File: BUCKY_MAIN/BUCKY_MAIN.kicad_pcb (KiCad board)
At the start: 2 copper layers, 190 x 162.2 mm, 17 parts, among them J2 MAG_CONN, J4 Conn_01x10, U1 IFX9201SG_BO, U2 IFX9201SG_BO, U3 IFX9201SG_BO, U9 PCA9548ADB

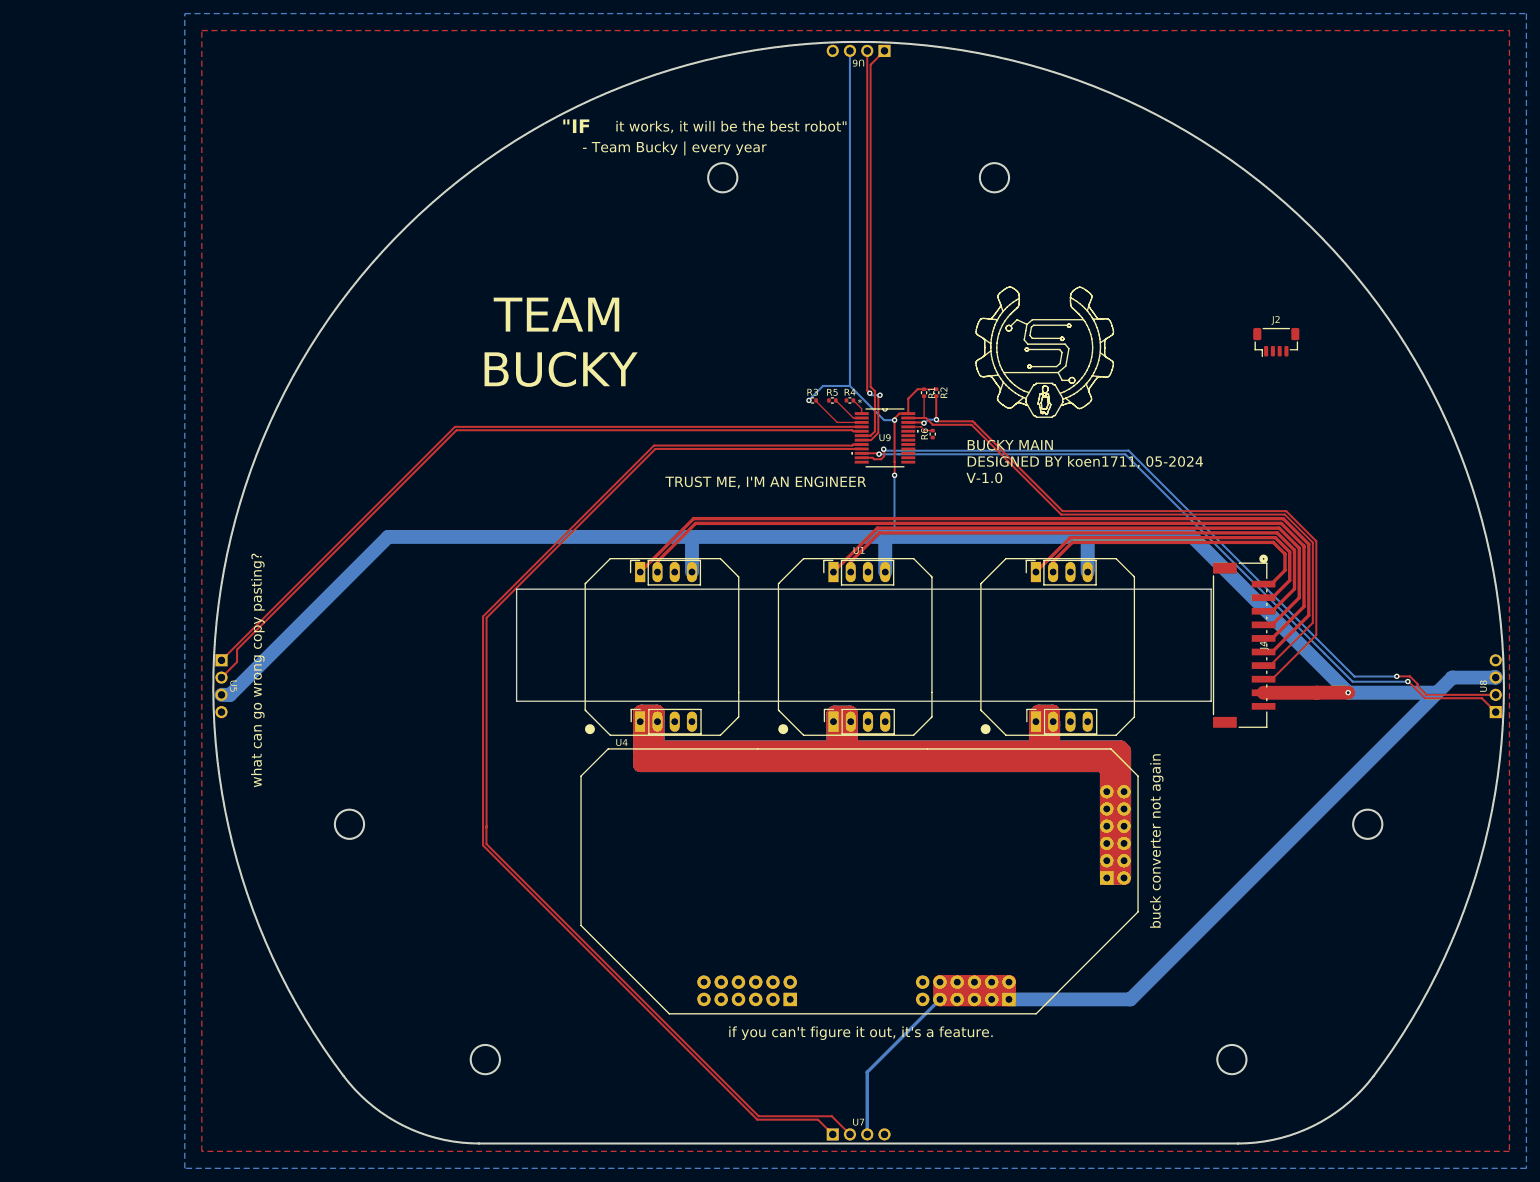
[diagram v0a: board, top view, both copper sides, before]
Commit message: chore: finish main board
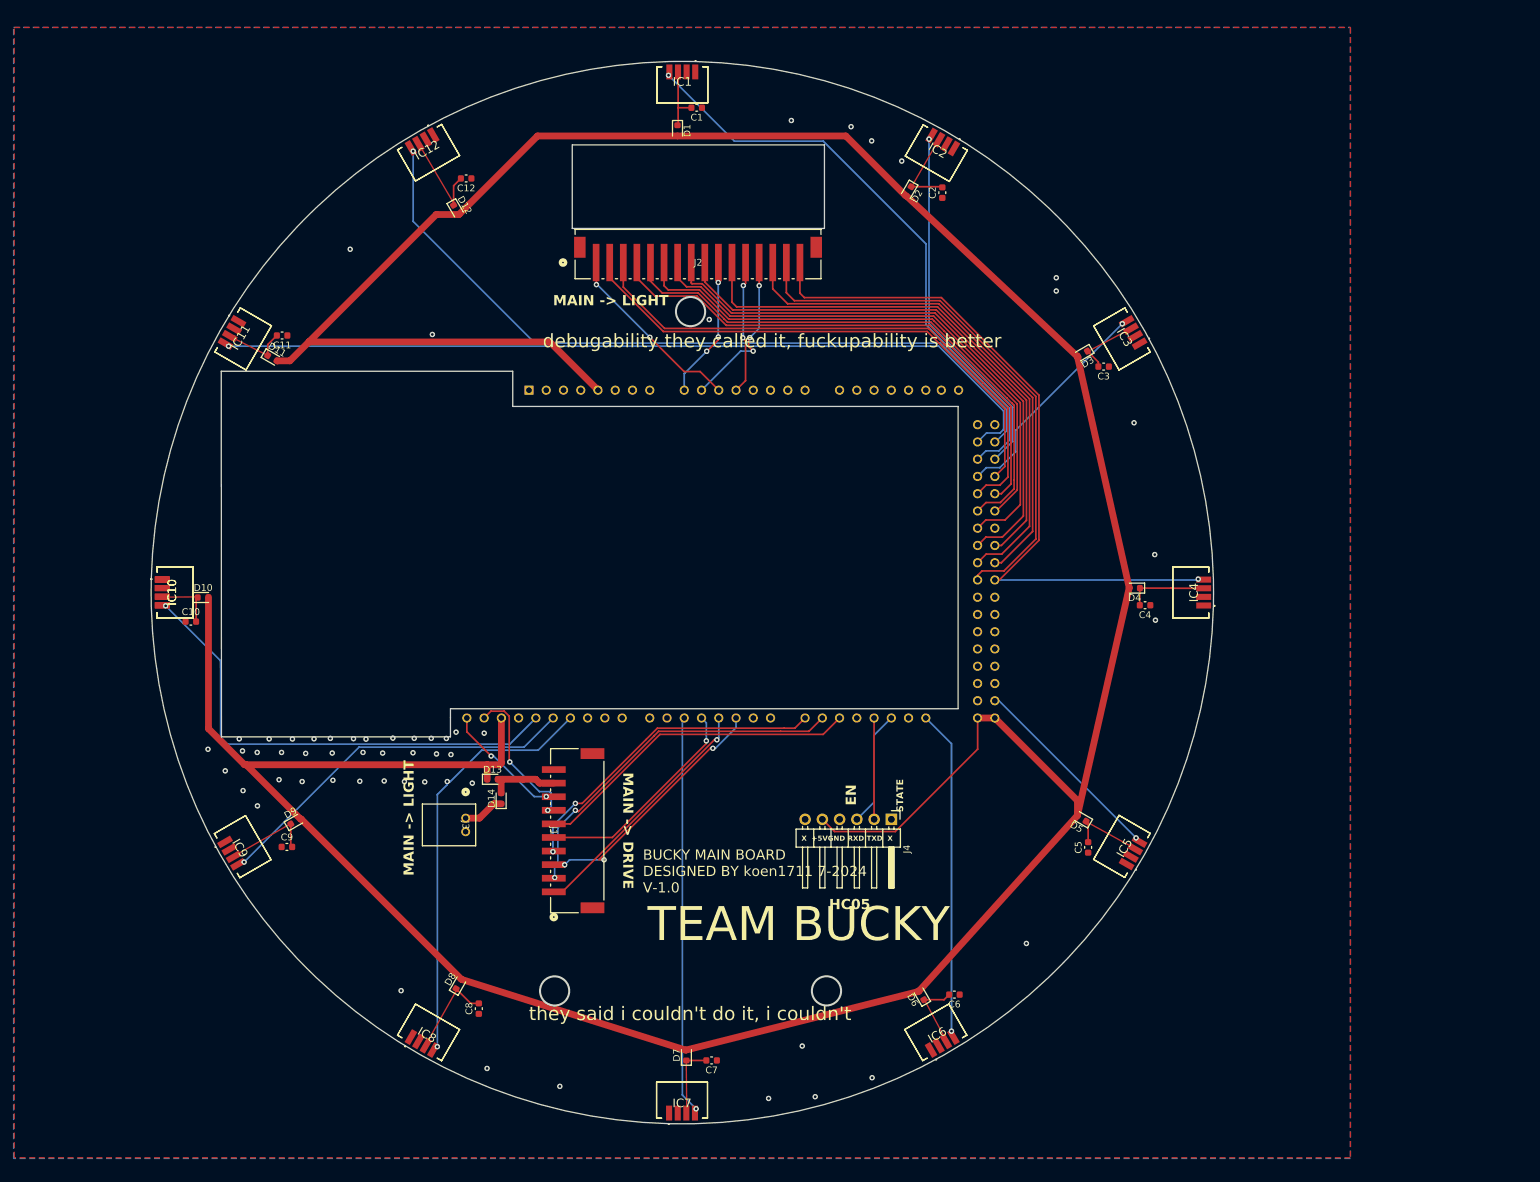
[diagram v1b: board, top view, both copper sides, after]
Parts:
- removed R1, R2: 4700R, Resistor_SMD:R_0402_1005Metric
- removed R3, R4, R5, R6: 10000R, Resistor_SMD:R_0402_1005Metric
- removed U1, U2, U3: IFX9201SG_BO, BUCKY_MAIN:IFX9201SG_BO
- removed U4: ~, BUCKY_MAIN:BUCKY_POWER
- removed U5, U6, U7, U8: ~, BUCKY_MAIN:BUCKY_TOF
- removed U9: PCA9548ADB, BUCKY_MAIN:DB24
- added A2: Arduino Mega, BUCKY_MAIN:ARDUINO_MEGA, B.Cu at (120.9, 92.3)
- added C1: 10uF, Capacitor_SMD:C_0603_1608Metric, F.Cu at (122.8, 26.6)
- added C10: 10uF, Capacitor_SMD:C_0603_1608Metric, F.Cu at (48.3, 102.3)
- added C11: 10uF, Capacitor_SMD:C_0603_1608Metric, F.Cu at (61.7, 60.1)
- added C12: 10uF, Capacitor_SMD:C_0603_1608Metric, F.Cu at (88.8, 37.0)
- added C2: 10uF, Capacitor_SMD:C_0603_1608Metric, F.Cu at (158.9, 39.1)
- added C3: 10uF, Capacitor_SMD:C_0603_1608Metric, F.Cu at (182.7, 64.7)
- added C4: 10uF, Capacitor_SMD:C_0603_1608Metric, F.Cu at (188.8, 99.9)
- added C5: 10uF, Capacitor_SMD:C_0603_1608Metric, F.Cu at (180.4, 135.5)
- added C6: 10uF, Capacitor_SMD:C_0603_1608Metric, F.Cu at (160.7, 157.2)
- added C7: 10uF, Capacitor_SMD:C_0603_1608Metric, F.Cu at (125.0, 166.9)
- added C8: 10uF, Capacitor_SMD:C_0603_1608Metric, F.Cu at (90.7, 159.2)
- added C9: 10uF, Capacitor_SMD:C_0603_1608Metric, F.Cu at (62.4, 135.4)
- added D1: D, Diode_SMD:D_0603_1608Metric, F.Cu at (119.9, 30.0)
- added D10: D, Diode_SMD:D_0603_1608Metric, F.Cu at (50.1, 98.7)
- added D11: D, Diode_SMD:D_0603_1608Metric, F.Cu at (60.3, 63.5)
- added D12: D, Diode_SMD:D_0603_1608Metric, F.Cu at (87.4, 41.7)
- added D13: D, Diode_SMD:D_0603_1608Metric, F.Cu at (92.7, 125.5)
- added D14: D, Diode_SMD:D_0603_1608Metric, F.Cu at (94.0, 128.3)
- added D2: D, Diode_SMD:D_0603_1608Metric, F.Cu at (153.9, 38.9)
- added D3: D, Diode_SMD:D_0603_1608Metric, F.Cu at (179.6, 62.8)
- added D4: D, Diode_SMD:D_0603_1608Metric, F.Cu at (187.2, 97.3)
- added D5: D, Diode_SMD:D_0603_1608Metric, F.Cu at (179.4, 131.3)
- added D6: D, Diode_SMD:D_0603_1608Metric, F.Cu at (155.8, 157.2)
- added D7: D, Diode_SMD:D_0603_1608Metric, F.Cu at (121.2, 166.1)
- added D8: D, Diode_SMD:D_0603_1608Metric, F.Cu at (87.7, 155.6)
- added D9: D, Diode_SMD:D_0603_1608Metric, F.Cu at (63.7, 131.7)
- added IC1: TSSP96038TR, BUCKY_MAIN:TSSP96038, F.Cu at (120.6, 23.2)
- added IC10 (x2): TSSP96038TR, BUCKY_MAIN:TSSP96038, F.Cu at (46.0, 98.0)
- added IC11: TSSP96038TR, BUCKY_MAIN:TSSP96038, F.Cu at (56.0, 60.7)
- added IC12: TSSP96038TR, BUCKY_MAIN:TSSP96038, F.Cu at (83.3, 33.2)
- added IC2: TSSP96038TR, BUCKY_MAIN:TSSP96038, F.Cu at (158.0, 33.3)
- added IC3: TSSP96038TR, BUCKY_MAIN:TSSP96038, F.Cu at (185.4, 60.7)
- added IC4: TSSP96038TR, BUCKY_MAIN:TSSP96038, F.Cu at (195.5, 98.0)
- added IC5: TSSP96038TR, BUCKY_MAIN:TSSP96038, F.Cu at (185.4, 135.4)
- added IC6: TSSP96038TR, BUCKY_MAIN:TSSP96038, F.Cu at (158.0, 162.7)
- added IC7: TSSP96038TR, BUCKY_MAIN:TSSP96038, F.Cu at (120.6, 172.7)
- added IC8: TSSP96038TR, BUCKY_MAIN:TSSP96038, F.Cu at (83.3, 162.7)
- added IC9: TSSP96038TR, BUCKY_MAIN:TSSP96038, F.Cu at (55.9, 135.4)
- added J1: Conn_01x10, BUCKY_MAIN:CONN10_S10B-PH_JST, F.Cu at (105.2, 133.1)
- added J3: Conn_01x02, BUCKY_MAIN:CONN_S2B-PH-K-S_JST, F.Cu at (88.7, 131.2)
- J2: value MAG_CONN -> Conn_01x16; footprint Connector_JST:JST_SH_BM04B-SRSS-TB_1x04-1MP_P1.00mm_Vertical -> BUCKY_MAIN:CONN_B16B-PH-SM4-TB_JST
- J4: value Conn_01x10 -> Conn_01x06; footprint BUCKY_MAIN:CONN10_S10B-PH_JST -> Connector_PinHeader_2.54mm:PinHeader_1x06_P2.54mm_Horizontal
- moved J2 86.1 mm to (123.0, 48.2)
- moved J4 57.4 mm to (151.4, 131.4), turned to -90 degrees
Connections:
- J2 pad 1: GND -> /R_A
- J2 pad 2: /SCL -> /R_S0
- J2 pad 3: /SDA -> /R_S1
- J2 pad 4: +3.3V -> /R_S2
- J4 pad 1: /M2_PWM -> /STATE
- J4 pad 2: /M2_DIR -> /TXD
- J4 pad 3: /M1_PWM -> /RXD
- J4 pad 4: /M1_DIR -> GND
- J4 pad 5: /M3_PWM -> +5V
- J4 pad 6: /M3_DIR -> /EN
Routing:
- net +12V: track 692.1 -> 0.00 mm
- net +5V: track 504.5 -> 295.4 mm, vias 4 -> 0
- net /SCL_2: track 170.1 -> 0.00 mm
- net /SDA_2: track 169.0 -> 0.00 mm
- net /IR_11: track 0.00 -> 125.4 mm, vias 0 -> 1
- net /IR_12: track 0.00 -> 114.7 mm, vias 0 -> 1
- net /SCL_3: track 111.0 -> 0.00 mm, vias 2 -> 0
- net /SCL_0: track 110.5 -> 0.00 mm
- net /SDA_3: track 109.5 -> 0.00 mm, vias 2 -> 0
- net /SDA_0: track 108.5 -> 0.00 mm
- net /IR_1: track 0.00 -> 88.1 mm, vias 0 -> 1
- net /M3_PWM: track 117.2 -> 32.2 mm, vias 0 -> 1
- net /D_S2: track 0.00 -> 84.5 mm
- net /F_S0: track 0.00 -> 84.2 mm
- net /R_S1: track 0.00 -> 83.3 mm
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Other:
- board size 190 x 162.2 mm -> 156.4 x 156.4 mm
- board text added: "BUCKY MAIN BOARD DESIGNED BY koen1711 7-2024 V-1.0"
- board text added: "EN"
- board text added: "HC05"
- board text added: "MAIN -> DRIVE"
- board text added: "MAIN -> LIGHT"
- board text added: "STATE"
- board text added: "X +5VGND RXD TXD X"
- board text added: "debugability they called it, fuckupability is better"
- board text added: "they said i couldn't do it, i couldn't"
- board text removed: "- Team Bucky | every year"
- board text removed: "BUCKY MAIN DESIGNED BY koen1711, 05-2024 V-1.0"
- board text removed: "JLCJLCJLCJLC"
- board text removed: "Mr Postma approves."
- board text removed: "TRUST ME, I'M AN ENGINEER"
- board text removed: "buck converter not again"
- board text removed: "if you can't figure it out, it's a feature."
- board text removed: "it works, it will be the best robot{dblquote}"
- board text removed: "what can go wrong copy pasting?"
- board text removed: "{dblquote}IF"
